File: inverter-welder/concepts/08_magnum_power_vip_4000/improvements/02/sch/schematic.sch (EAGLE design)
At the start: 13 parts, among them P1 50k B

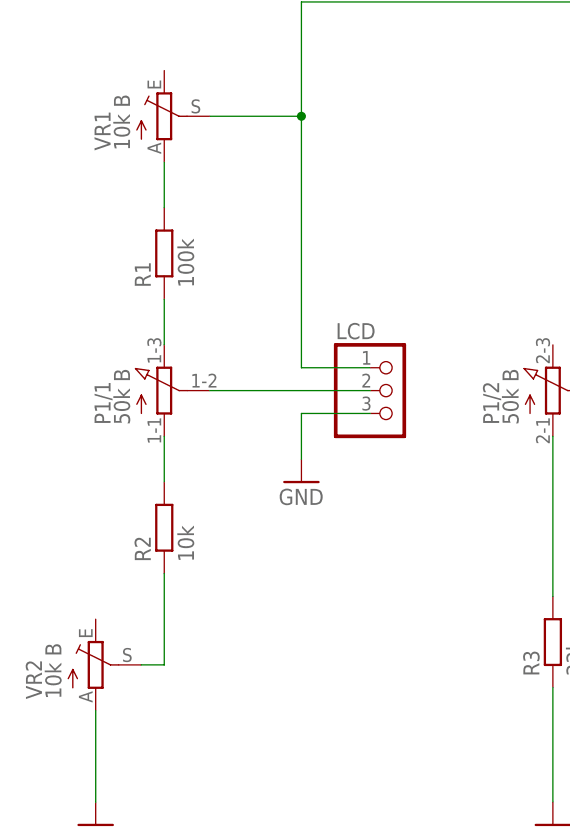
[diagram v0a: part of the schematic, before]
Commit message: [Welder] More work in the topic.
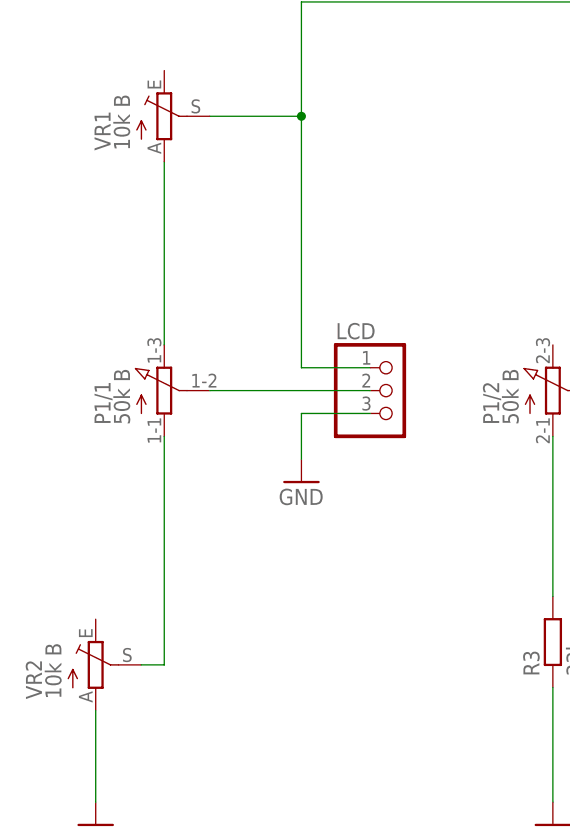
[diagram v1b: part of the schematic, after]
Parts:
- removed R1: 100k, rcl:R-EU_0204/5
- removed R2: 10k, rcl:R-EU_0204/5
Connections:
- removed net N$5: P1/1.E, R1.1
- removed net N$9: R2.1, VR2.S
- net N$4: now also VR2.S; no longer R2.2
- net N$7: now also P1/1.E; no longer R1.2
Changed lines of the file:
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@@
 <part name="LCD" library="pinhead" library_urn="urn:adsk.eagle:library:325" deviceset="PINHD-1X3" device="" package3d_urn="urn:adsk.eagle:package:22458/2"/>
 <part name="GND3" library="supply1" library_urn="urn:adsk.eagle:library:371" deviceset="GND" device=""/>
-<part name="R1" library="rcl" library_urn="urn:adsk.eagle:library:334" deviceset="R-EU_" device="0204/5" package3d_urn="urn:adsk.eagle:package:23488/1" value="100k"/>
-<part name="R2" library="rcl" library_urn="urn:adsk.eagle:library:334" deviceset="R-EU_" device="0204/5" package3d_urn="urn:adsk.eagle:package:23488/1" value="10k"/>
 <part name="S1" library="switch" library_urn="urn:adsk.eagle:library:380" deviceset="CK10" device="" package3d_urn="urn:adsk.eagle:package:27744/1"/>
 <part name="PIN8" library="pinhead" library_urn="urn:adsk.eagle:library:325" deviceset="PINHD-1X1" device="" package3d_urn="urn:adsk.eagle:package:22485/2"/>
@@
 <instance part="GND3" gate="1" x="60.96" y="40.64" smashed="yes">
 <attribute name="VALUE" x="58.42" y="38.1" size="1.778" layer="96"/>
-</instance>
-<instance part="R1" gate="G$1" x="45.72" y="66.04" smashed="yes" rot="R90">
-<attribute name="NAME" x="44.2214" y="62.23" size="1.778" layer="95" rot="R90"/>
-<attribute name="VALUE" x="49.022" y="62.23" size="1.778" layer="96" rot="R90"/>
-</instance>
-<instance part="R2" gate="G$1" x="45.72" y="35.56" smashed="yes" rot="R90">
-<attribute name="NAME" x="44.2214" y="31.75" size="1.778" layer="95" rot="R90"/>
-<attribute name="VALUE" x="49.022" y="31.75" size="1.778" layer="96" rot="R90"/>
 </instance>
 <instance part="S1" gate="G$1" x="132.08" y="83.82" smashed="yes" rot="R270">
@@
 </segment>
 </net>
-<net name="N$5" class="0">
-<segment>
-<pinref part="P1" gate="/1" pin="E"/>
-<pinref part="R1" gate="G$1" pin="1"/>
-<wire x1="45.72" y1="55.88" x2="45.72" y2="60.96" width="0.1524" layer="91"/>
-</segment>
-</net>
 <net name="N$7" class="0">
 <segment>
-<pinref part="R1" gate="G$1" pin="2"/>
 <pinref part="VR1" gate="1" pin="A"/>
-<wire x1="45.72" y1="71.12" x2="45.72" y2="76.2" width="0.1524" layer="91"/>
+<pinref part="P1" gate="/1" pin="E"/>
+<wire x1="45.72" y1="76.2" x2="45.72" y2="55.88" width="0.1524" layer="91"/>
 </segment>
 </net>
@@
 <segment>
 <pinref part="P1" gate="/1" pin="A"/>
-<pinref part="R2" gate="G$1" pin="2"/>
-<wire x1="45.72" y1="45.72" x2="45.72" y2="40.64" width="0.1524" layer="91"/>
+<pinref part="VR2" gate="1" pin="S"/>
+<wire x1="43.18" y1="20.32" x2="45.72" y2="20.32" width="0.1524" layer="91"/>
+<wire x1="45.72" y1="45.72" x2="45.72" y2="20.32" width="0.1524" layer="91"/>
 </segment>
 </net>
-<net name="N$9" class="0">
-<segment>
-<pinref part="VR2" gate="1" pin="S"/>
-<pinref part="R2" gate="G$1" pin="1"/>
-<wire x1="43.18" y1="20.32" x2="45.72" y2="20.32" width="0.1524" layer="91"/>
-<wire x1="45.72" y1="20.32" x2="45.72" y2="30.48" width="0.1524" layer="91"/>
-</segment>
-</net>
